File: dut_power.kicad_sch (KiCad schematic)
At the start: 51 parts, among them J10 Conn_01x04, J6 Conn_02x04_Odd_Even, J7 Conn_01x02, J8 Conn_02x04_Odd_Even, J9 Conn_02x04_Odd_Even, Q1 AO3401A, U1 TCA9535PWR(UMW)

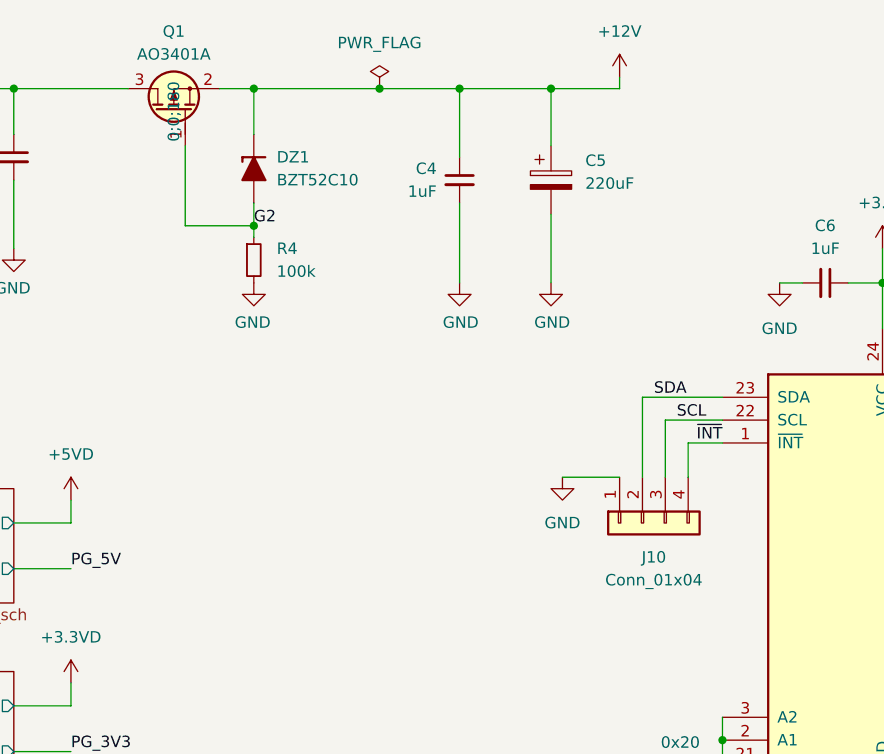
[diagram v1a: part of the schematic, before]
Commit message: WIP v0.2.0 changes
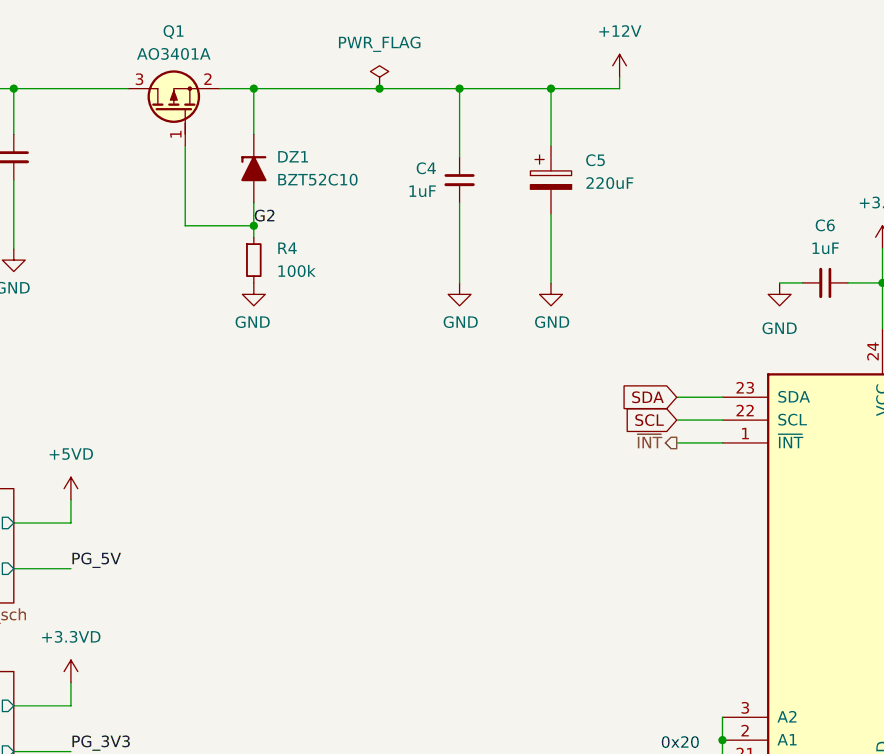
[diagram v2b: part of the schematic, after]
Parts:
- removed J10: Conn_01x04, HL_Connector_Pad_2.54mm:Pad_1x04_P2.54_1.7x1.7_Rect-Oct, symbol Connector_Generic:Conn_01x04
- J7: footprint Connector_Phoenix_MC:PhoenixContact_MCV_1,5_2-G-3.81_1x02_P3.81mm_Vertical -> Connector_Phoenix_MC:PhoenixContact_MC_1,5_2-G-3.81_1x02_P3.81mm_Horizontal; JLCPCB_CORRECTION 1.905;0;180 -> (none); LCSC (none) -> C8387; THT_LCSC C8396 -> (none)
